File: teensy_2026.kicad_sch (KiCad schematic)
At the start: 20 parts, among them J1 LED, J10 Strain Gauge, J11 Strain Gauge, J12 Strain Gauge, J15 LinAct1, J2 BattManagement, J3 LinearActSaber, J4 Current Sense, J5 LinAct2, J6 Current Sense, J7 Current Sense, J8 Strain Gauge, J9 Strain Gauge, U1 RASPBERRY_PI_PICO

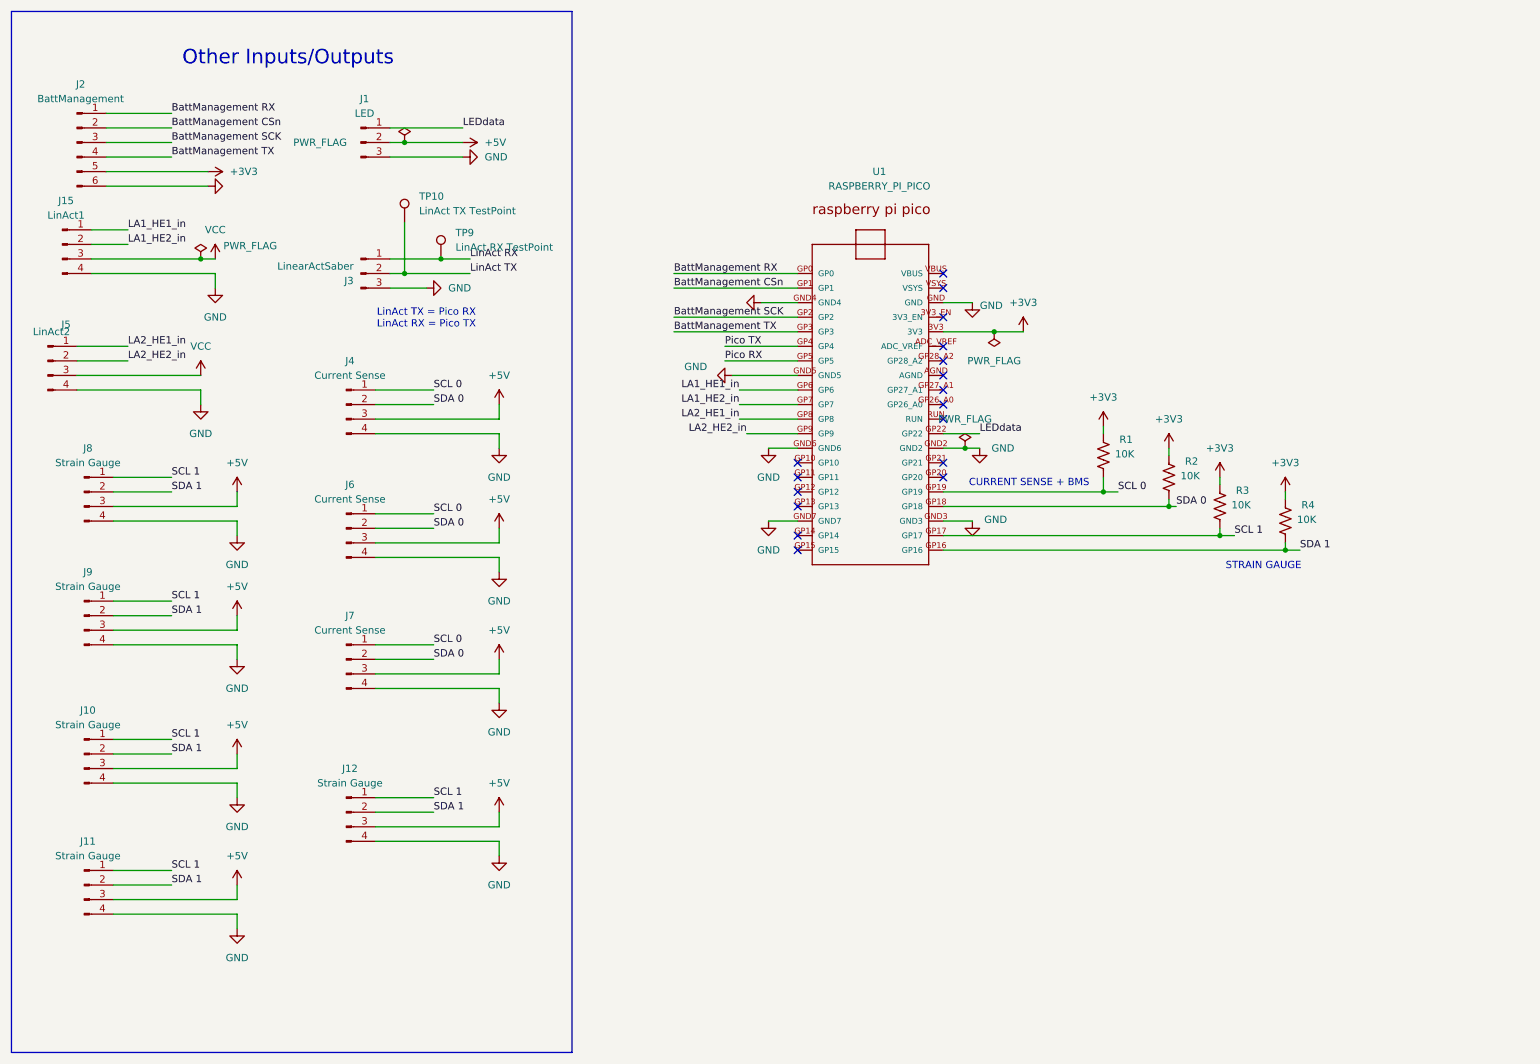
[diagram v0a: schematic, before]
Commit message: Extra UART
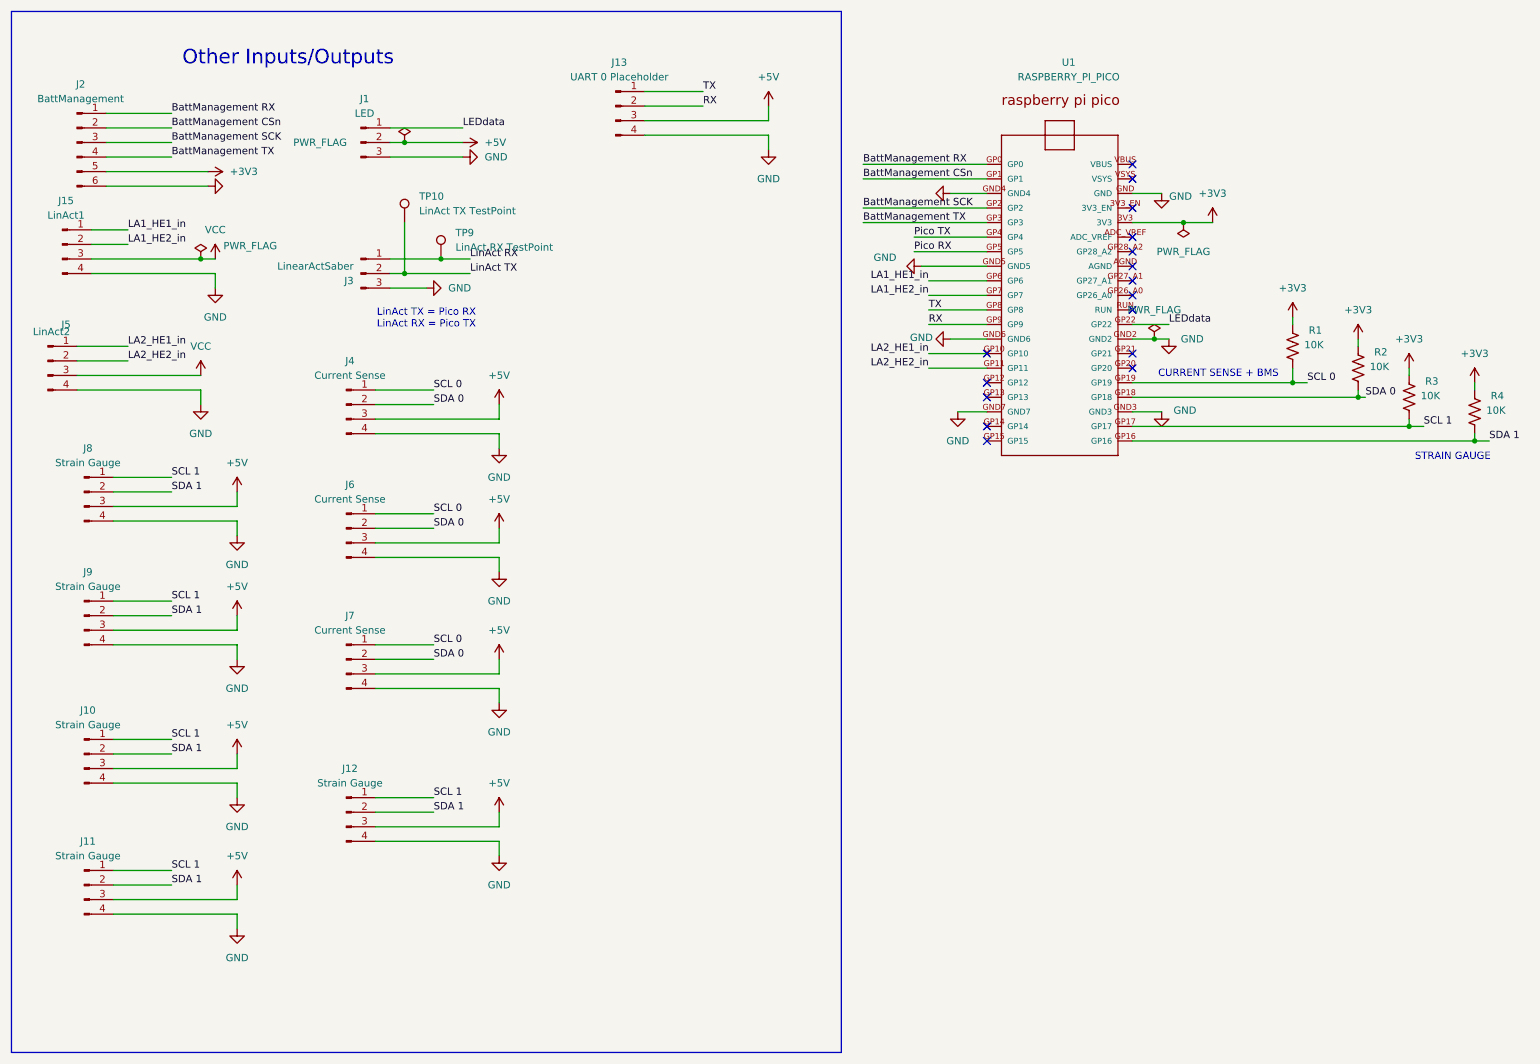
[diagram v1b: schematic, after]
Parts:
- added J13: UART 0 Placeholder, symbol Connector:Conn_01x04_Pin
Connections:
- net +5V: now also J13.3 (Pin_3)
- net GND: now also J13.4 (Pin_4)
- net LA2_HE1_in: now also U1.GP10; no longer U1.GP8
- net LA2_HE2_in: now also U1.GP11; no longer U1.GP9
- new net RX: J13.2 (Pin_2), U1.GP9
- new net TX: J13.1 (Pin_1), U1.GP8
- no-connect marks 17 -> 16
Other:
- moved on the sheet: R1, R2, R3, R4, U1
